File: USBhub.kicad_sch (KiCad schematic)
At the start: 20 parts, among them J10 482040001, J4 482040001, J5 482040001, J6 482040001, U10 FE1.1s, U11 24LC02B-I_SN, Y3 ABLS-12.000MHZ-B2-T

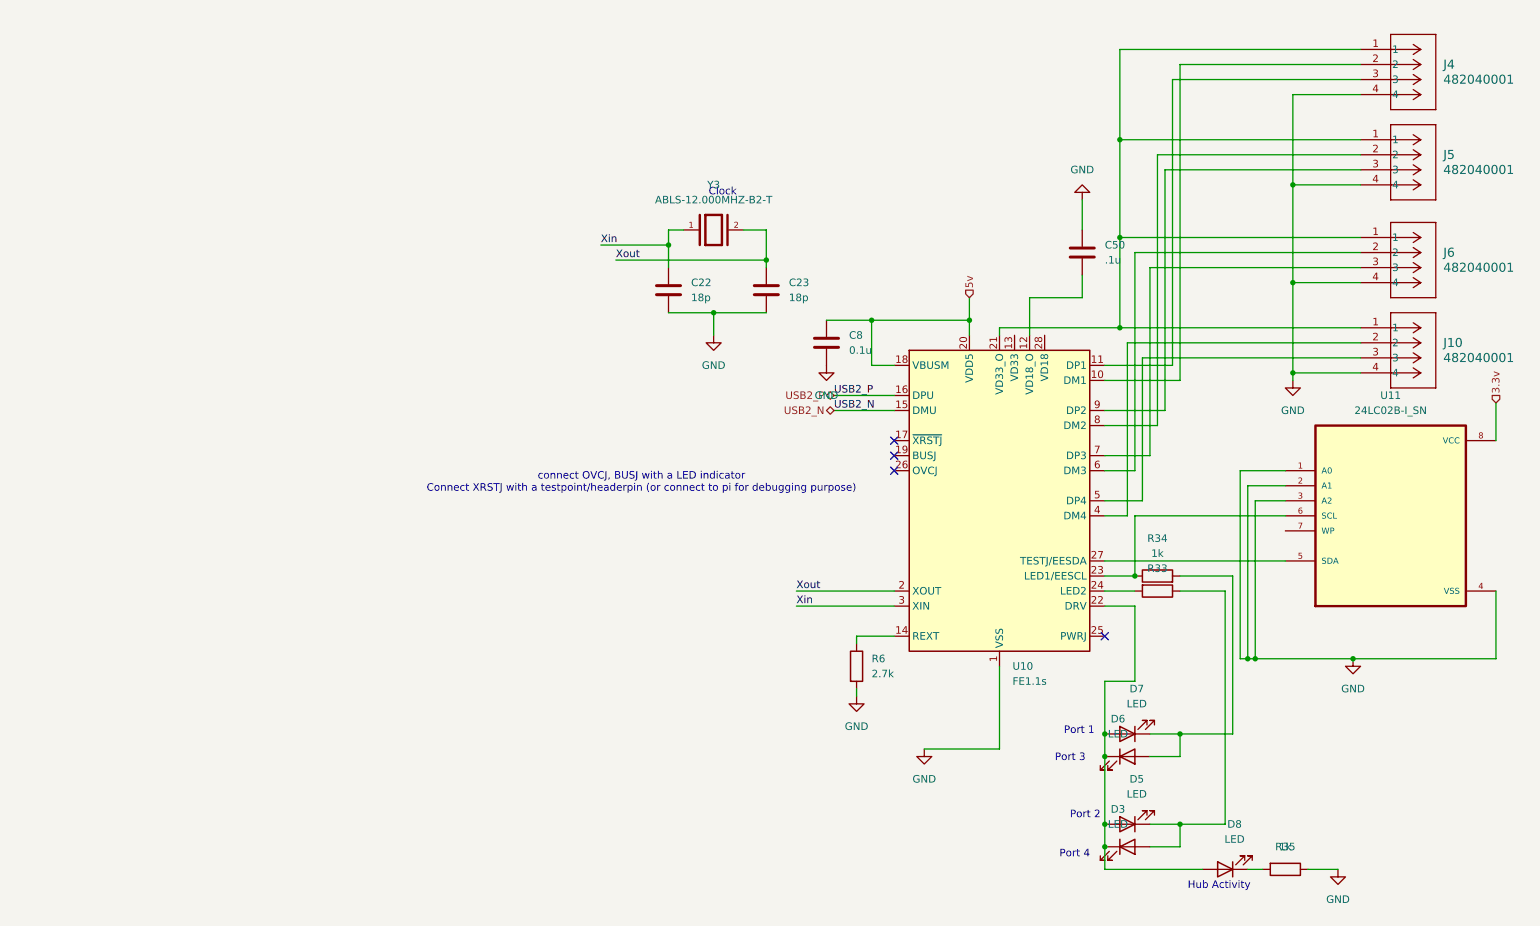
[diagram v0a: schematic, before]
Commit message: stuff
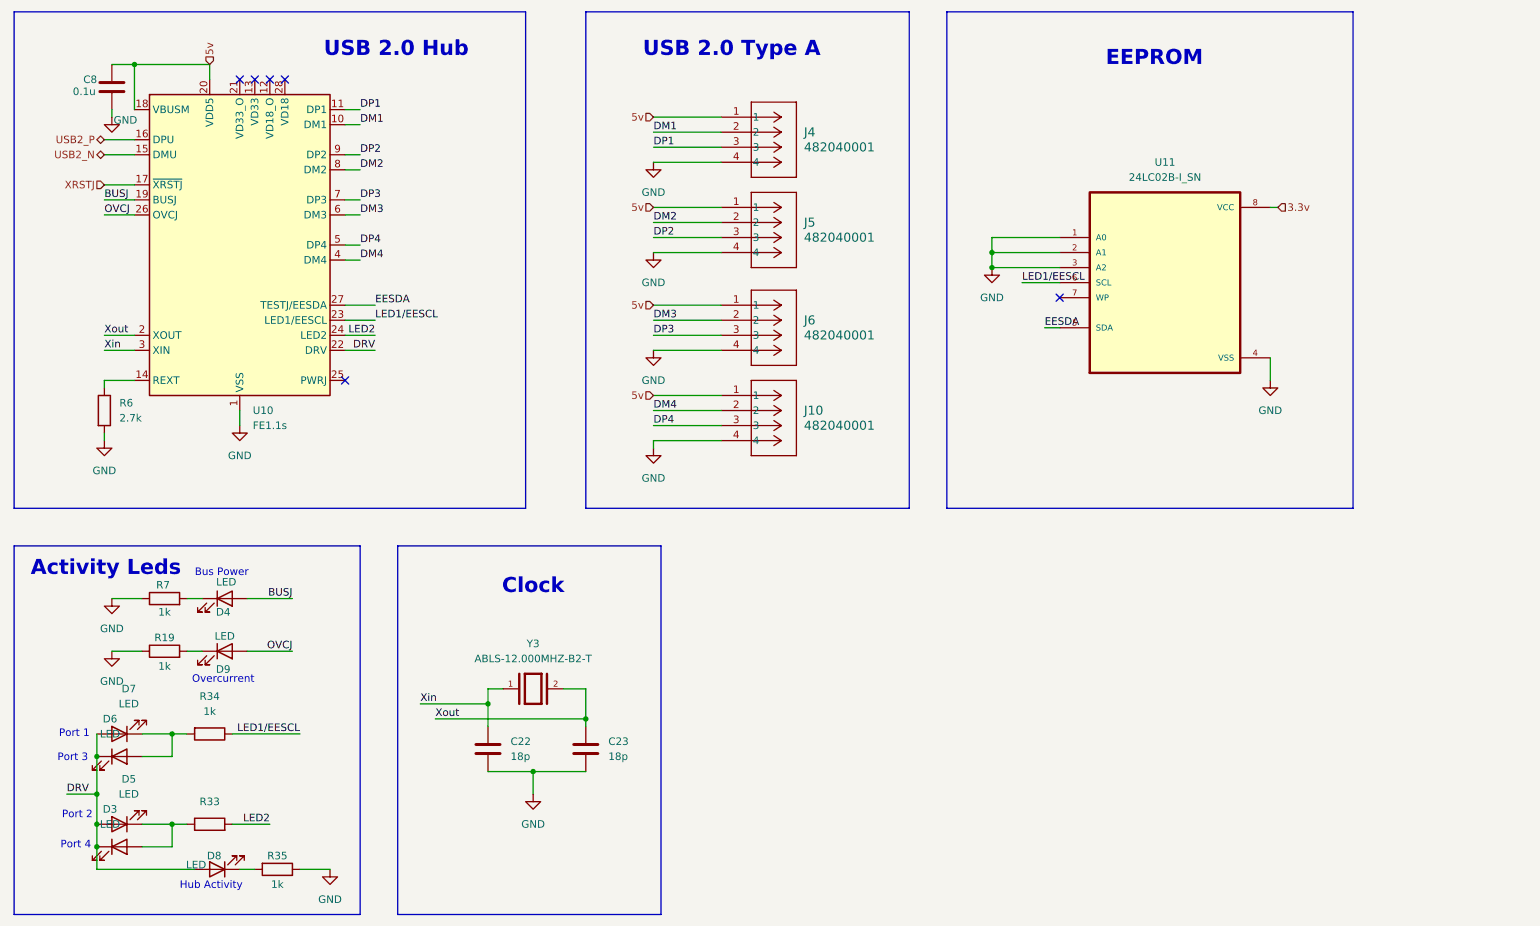
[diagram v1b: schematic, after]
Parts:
- removed C50: .1u, symbol Device:C
- added D4, D9: LED, symbol Device:LED
- added R19, R7: 1k, symbol Device:R
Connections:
- net 5v: now also J10.1, J4.1, J5.1, J6.1
- net GND: now also R19.1, R7.1
- net DRV: now reaches D3.1 (K), D5.2 (A), D6.1 (K), D7.2 (A), D8.2 (A), U10.22 (DRV)
- net DM1: now reaches J4.2, U10.10 (DM1)
- net DP1: now reaches J4.3, U10.11 (DP1)
- net LED1/EESCL: now reaches R34.1, U10.23 (LED1/EESCL), U11.6 (SCL)
- net LED2: now reaches R33.2, U10.24 (LED2)
- net DM2: now reaches J5.2, U10.8 (DM2)
- net DP2: now reaches J5.3, U10.9 (DP2)
- net DM4: now reaches J10.2, U10.4 (DM4)
- net DP4: now reaches J10.3, U10.5 (DP4)
- net EESDA: now reaches U10.27 (TESTJ/EESDA), U11.5 (SDA)
- net DM3: now reaches J6.2, U10.6 (DM3)
- net DP3: now reaches J6.3, U10.7 (DP3)
- net XRSTJ: now reaches U10.17 (~{XRSTJ})
- net BUSJ: now reaches U10.19 (BUSJ)
- net BUSJ: now also D4.2 (A)
- net OVCJ: now reaches U10.26 (OVCJ)
- net OVCJ: now also D9.2 (A)
- new net: D9.1 (K), R19.2
- new net: D4.1 (K), R7.2
- now unconnected: U10.21 (VD33_O)
- no-connect marks 4 -> 6
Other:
- note added: "Activity Leds"
- note added: "Bus Power"
- note added: "EEPROM"
- note added: "Overcurrent"
- note added: "USB 2.0 Hub"
- note added: "USB 2.0 Type A"
- note removed: "connect OVCJ, BUSJ with a LED indicator Connect XRSTJ with a testpoint/headerpin (or connect to pi for debugging purpose)"
- moved on the sheet: C22, C23, C8, D3, D5, D6, D7, D8, J10, J4, J5, J6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
